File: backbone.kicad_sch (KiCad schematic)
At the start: 6 parts

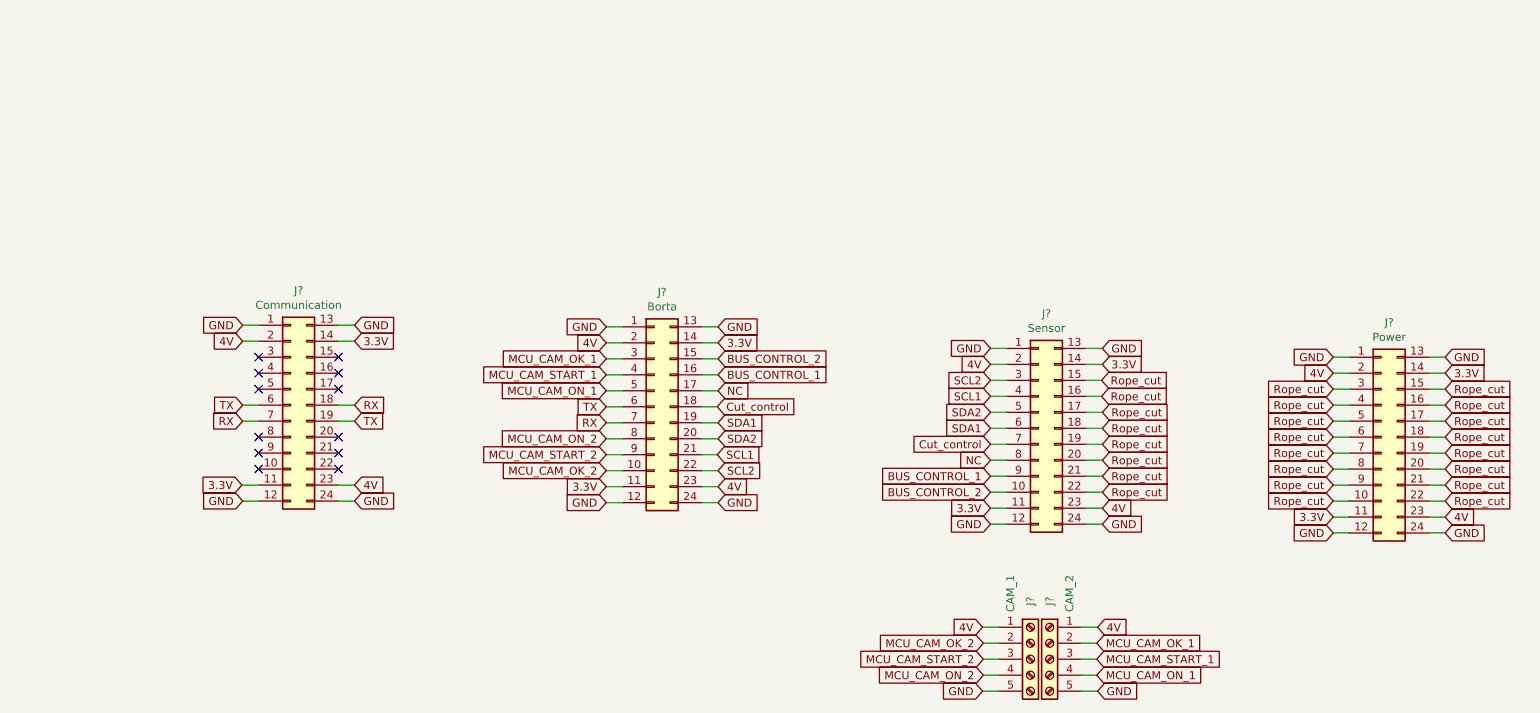
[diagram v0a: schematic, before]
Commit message: 0.1v
Ridiculess backbone
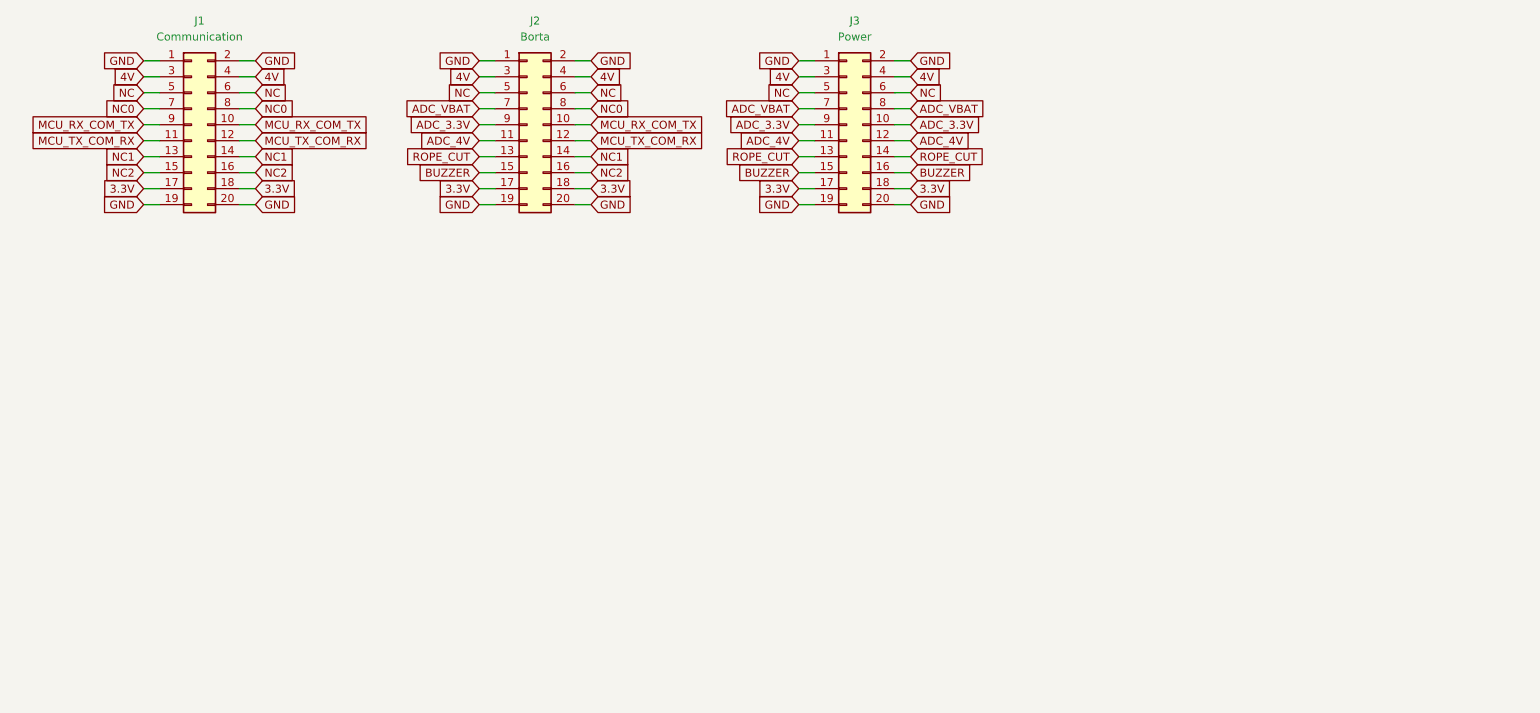
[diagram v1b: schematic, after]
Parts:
- removed J?: Borta, LOCAL:PinHeader_2x12_P2.54mm_Vertical, symbol Connector_Generic:Conn_02x12_Top_Bottom
- removed J?: CAM_2, 5_pin_connector:HDRV5W114P0X396_1X5_1974X850X1070P, symbol Connector:Screw_Terminal_01x05
- removed J?: Power, LOCAL:PinHeader_2x12_P2.54mm_Vertical, symbol Connector_Generic:Conn_02x12_Top_Bottom
- removed J?: Sensor, LOCAL:PinHeader_2x12_P2.54mm_Vertical, symbol Connector_Generic:Conn_02x12_Top_Bottom
- removed J?: Communication, LOCAL:PinHeader_2x12_P2.54mm_Vertical, symbol Connector_Generic:Conn_02x12_Top_Bottom
- removed J?: CAM_1, 5_pin_connector:HDRV5W114P0X396_1X5_1974X850X1070P, symbol Connector:Screw_Terminal_01x05
- added J1: Communication, Connector_PinSocket_2.54mm:PinSocket_2x10_P2.54mm_Vertical, symbol Connector_Generic:Conn_02x10_Odd_Even
- added J2: Borta, Connector_PinSocket_2.54mm:PinSocket_2x10_P2.54mm_Vertical, symbol Connector_Generic:Conn_02x10_Odd_Even
- added J3: Power, Connector_PinSocket_2.54mm:PinSocket_2x10_P2.54mm_Vertical, symbol Connector_Generic:Conn_02x10_Odd_Even
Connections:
- net 3.3V: now also J1.17 (Pin_17), J1.18 (Pin_18), J2.17 (Pin_17), J2.18 (Pin_18), J3.17 (Pin_17), J3.18 (Pin_18)
- net 4V: now also J1.3 (Pin_3), J1.4 (Pin_4), J2.3 (Pin_3), J2.4 (Pin_4), J3.3 (Pin_3), J3.4 (Pin_4)
- net GND: now also J1.1 (Pin_1), J1.19 (Pin_19), J1.2 (Pin_2), J1.20 (Pin_20), J2.1 (Pin_1), J2.19 (Pin_19), J2.2 (Pin_2), J2.20 (Pin_20), J3.1 (Pin_1), J3.19 (Pin_19), J3.2 (Pin_2), J3.20 (Pin_20)
- net NC: now also J1.5 (Pin_5), J1.6 (Pin_6), J2.5 (Pin_5), J2.6 (Pin_6), J3.5 (Pin_5), J3.6 (Pin_6)
- new net ADC_3.3V: J2.9 (Pin_9), J3.10 (Pin_10), J3.9 (Pin_9)
- new net ADC_4V: J2.11 (Pin_11), J3.11 (Pin_11), J3.12 (Pin_12)
- new net ADC_VBAT: J2.7 (Pin_7), J3.7 (Pin_7), J3.8 (Pin_8)
- new net BUZZER: J2.15 (Pin_15), J3.15 (Pin_15), J3.16 (Pin_16)
- new net MCU_RX_COM_TX: J1.10 (Pin_10), J1.9 (Pin_9), J2.10 (Pin_10)
- new net MCU_TX_COM_RX: J1.11 (Pin_11), J1.12 (Pin_12), J2.12 (Pin_12)
- new net NC0: J1.7 (Pin_7), J1.8 (Pin_8), J2.8 (Pin_8)
- new net NC1: J1.13 (Pin_13), J1.14 (Pin_14), J2.14 (Pin_14)
- new net NC2: J1.15 (Pin_15), J1.16 (Pin_16), J2.16 (Pin_16)
- new net ROPE_CUT: J2.13 (Pin_13), J3.13 (Pin_13), J3.14 (Pin_14)
- no-connect marks 12 -> 0
